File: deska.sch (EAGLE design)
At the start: 12 parts, among them IC1 78L05Z, T1 TIP122, T2 TIP122, T3 TIP122

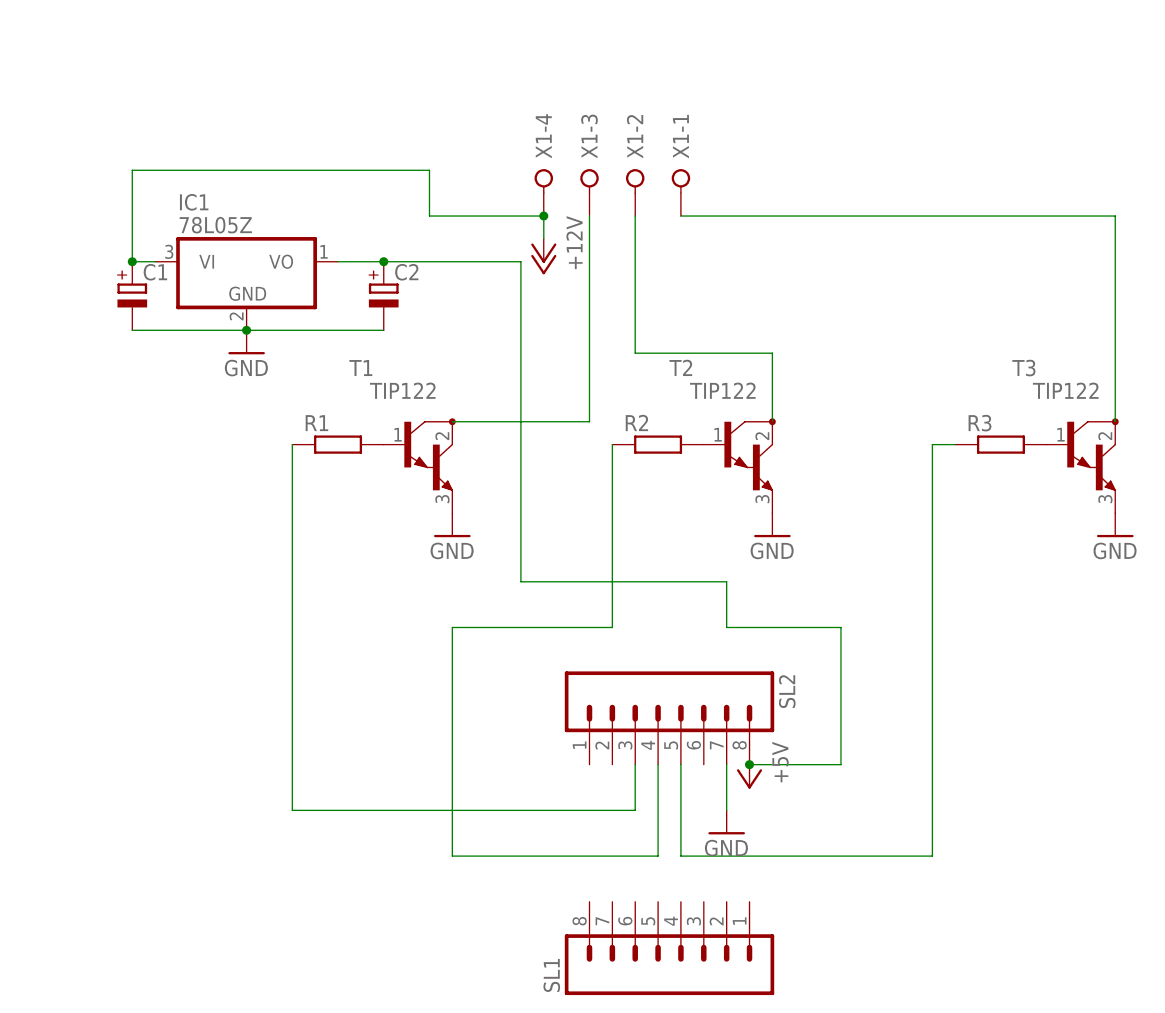
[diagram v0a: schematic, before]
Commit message: verze ESP8266-01
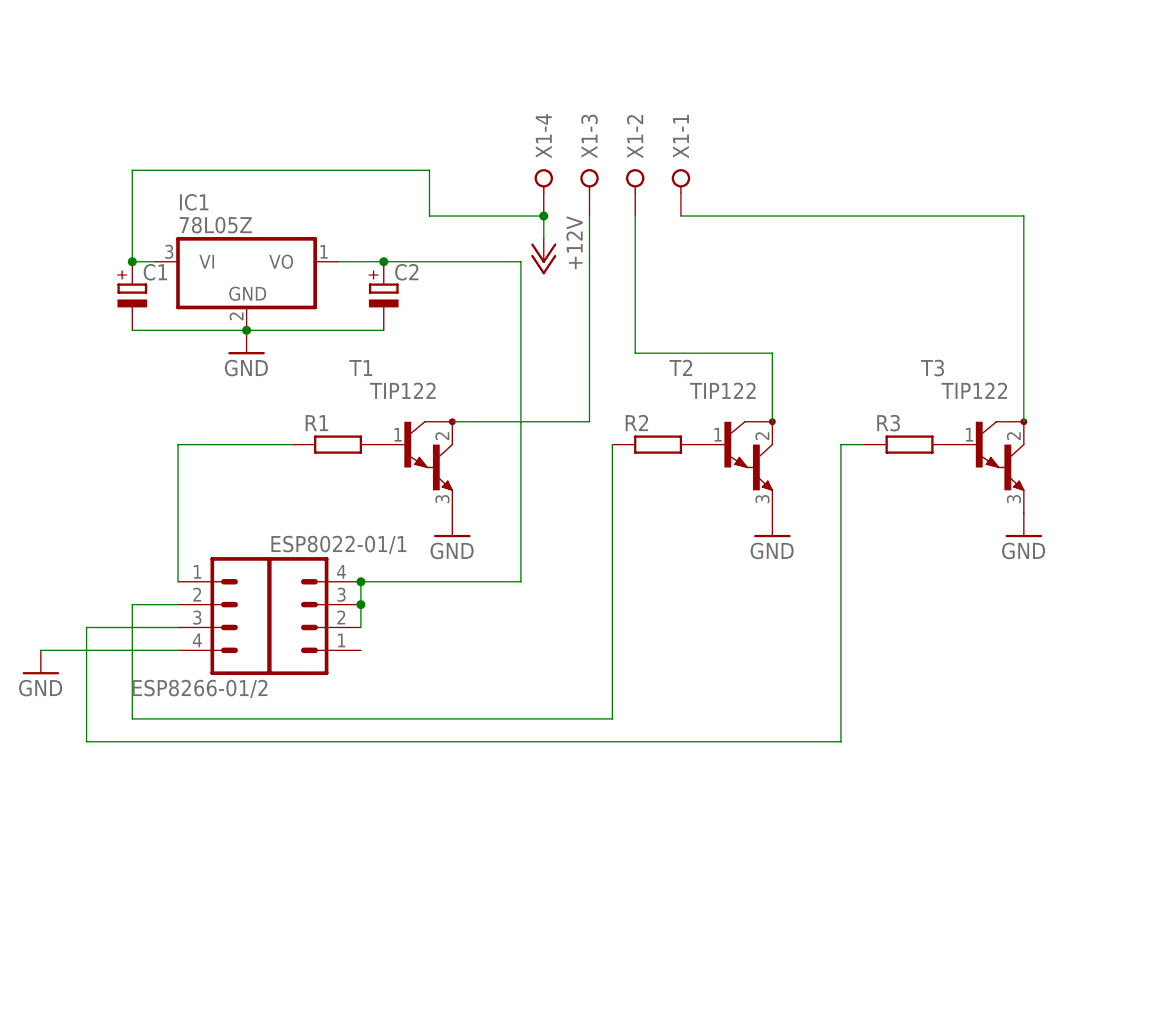
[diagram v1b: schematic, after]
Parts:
- removed SL1, SL2: (no value), con-amp-quick:M08
- added ESP8022-01/1, ESP8266-01/2: (no value), con-amp-quick:M04
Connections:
- removed net +5V: C2.+, IC1.VO, SL2.8
- removed net N$9: R3.1, SL2.5
- new net N$10: ESP8266-01/2.3, R3.1
- new net N$11: C2.+, ESP8022-01/1.2, ESP8022-01/1.3, ESP8022-01/1.4, IC1.VO
- net GND: now also ESP8266-01/2.4; no longer SL2.7
- net N$7: now also ESP8266-01/2.1; no longer SL2.3
- net N$8: now also ESP8266-01/2.2; no longer SL2.4
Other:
- moved on the sheet: R3, T3

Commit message: zmeny plosnaku
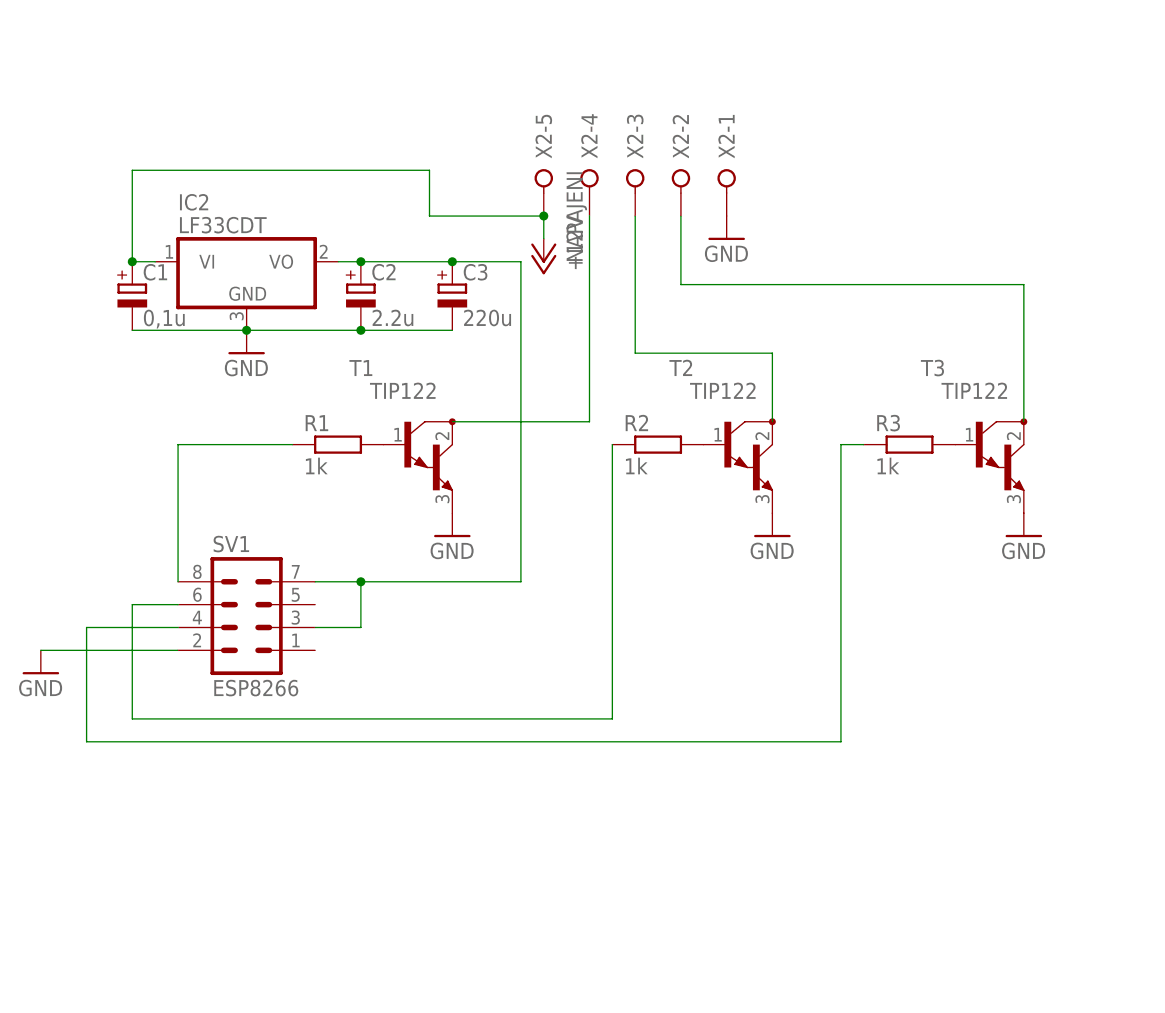
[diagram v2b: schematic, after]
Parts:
- removed ESP8022-01/1, ESP8266-01/2: (no value), con-amp-quick:M04
- removed IC1: 78L05Z, linear:78L05Z
- removed X1: (no value), con-wago-508:W237-04P
- added C3: 220u, rcl:CPOL-EUE3.5-8
- added IC2: LF33CDT, linear:7805DT
- added SV1: ESP8266, con-lstb:MA04-2
- added X2: NAPAJENI, con-wago-508:W237-05P
- C1: value (none) -> 0,1u
- C2: value (none) -> 2.2u
- R1, R2, R3: value (none) -> 1k
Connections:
- net +12V: now also IC2.VI, X2-5.KL; no longer IC1.VI, X1-4.KL
- net GND: now also C3.-, IC2.GND, SV1.2, X2-1.KL; no longer ESP8266-01/2.4, IC1.GND
- net N$1: now also X2-4.KL; no longer X1-3.KL
- net N$10: now also SV1.4; no longer ESP8266-01/2.3
- net N$11: now also C3.+, IC2.VO, SV1.3, SV1.7; no longer ESP8022-01/1.2, ESP8022-01/1.3, ESP8022-01/1.4, IC1.VO
- net N$2: now also X2-3.KL; no longer X1-2.KL
- net N$3: now also X2-2.KL; no longer X1-1.KL
- net N$7: now also SV1.8; no longer ESP8266-01/2.1
- net N$8: now also SV1.6; no longer ESP8266-01/2.2
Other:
- moved on the sheet: C2

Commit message: uprava desky
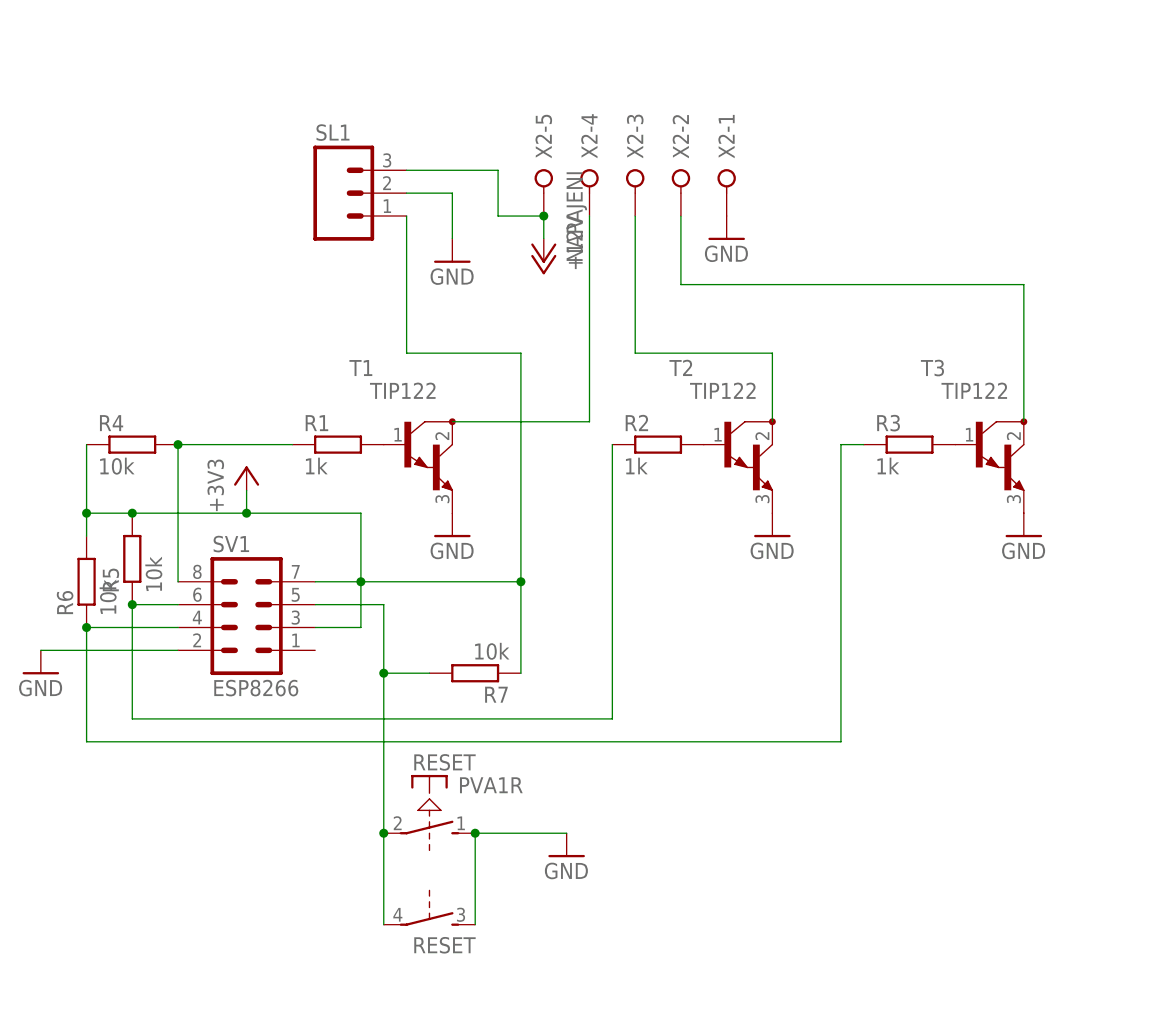
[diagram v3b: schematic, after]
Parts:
- removed C1: 0,1u, rcl:CPOL-EUE2-5
- removed C2: 2.2u, rcl:CPOL-EUE2-5
- removed C3: 220u, rcl:CPOL-EUE3.5-8
- removed IC2: LF33CDT, linear:7805DT
- added R4, R5, R6, R7: 10k, rcl:R-EU_0207/10
- added RESET: PVA1R, switch-misc:PVA1R
- added SL1: (no value), con-amp-quick:M03
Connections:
- removed net N$11: C2.+, C3.+, IC2.VO, SV1.3, SV1.7
- new net +3V3: R4.1, R5.2, R6.2, R7.1, SL1.1, SV1.3, SV1.7
- new net N$12: R7.2, RESET1.P, RESET2.P, SV1.5
- net +12V: now also SL1.3; no longer C1.+, IC2.VI
- net GND: now also RESET1.S, RESET2.S, SL1.2; no longer C1.-, C2.-, C3.-, IC2.GND
- net N$10: now also R6.1
- net N$7: now also R4.2
- net N$8: now also R5.1
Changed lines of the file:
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@@
 <?xml version="1.0" encoding="utf-8"?>
 <!DOCTYPE eagle SYSTEM "eagle.dtd">
-<eagle version="7.7.0">
+<eagle version="9.1.3">
 <drawing>
 <settings>
 <setting alwaysvectorfont="no"/>
+<setting keepoldvectorfont="yes"/>
 <setting verticaltext="up"/>
 </settings>
@@
 <part name="R2" library="rcl" deviceset="R-EU_" device="0207/10" value="1k"/>
 <part name="R3" library="rcl" deviceset="R-EU_" device="0207/10" value="1k"/>
-<part name="GND5" library="supply1" deviceset="GND" device=""/>
 <part name="GND6" library="supply1" deviceset="GND" device=""/>
-<part name="C3" library="rcl" deviceset="CPOL-EU" device="E3.5-8" value="220u"/>
-<part name="IC2" library="linear" deviceset="78*" device="DT" technology="05" value="LF33CDT"/>
 <part name="X2" library="con-wago-508" deviceset="W237-05P" device="" value="NAPAJENI"/>
 <part name="GND4" library="supply1" deviceset="GND" device=""/>
-<part name="C1" library="rcl" deviceset="CPOL-EU" device="E2-5" value="0,1u"/>
-<part name="C2" library="rcl" deviceset="CPOL-EU" device="E2-5" value="2.2u"/>
 <part name="SV1" library="con-lstb" deviceset="MA04-2" device="" value="ESP8266"/>
+<part name="R4" library="rcl" deviceset="R-EU_" device="0207/10" value="10k"/>
+<part name="R5" library="rcl" deviceset="R-EU_" device="0207/10" value="10k"/>
+<part name="R6" library="rcl" deviceset="R-EU_" device="0207/10" value="10k"/>
+<part name="R7" library="rcl" deviceset="R-EU_" device="0207/10" value="10k"/>
+<part name="RESET" library="switch-misc" library_urn="urn:adsk.eagle:library:376" deviceset="PVA1R" device="" package3d_urn="urn:adsk.eagle:package:27429/1"/>
+<part name="GND7" library="supply1" deviceset="GND" device=""/>
+<part name="+3V1" library="supply1" library_urn="urn:adsk.eagle:library:371" deviceset="+3V3" device=""/>
+<part name="SL1" library="con-amp-quick" library_urn="urn:adsk.eagle:library:125" deviceset="M03" device="" package3d_urn="urn:adsk.eagle:package:5957/1"/>
+<part name="GND5" library="supply1" deviceset="GND" device=""/>
 </parts>
 <sheets>
@@
 <instance part="R2" gate="G$1" x="45.72" y="66.04"/>
 <instance part="R3" gate="G$1" x="73.66" y="66.04"/>
-<instance part="GND5" gate="1" x="0" y="76.2"/>
 <instance part="GND6" gate="1" x="-22.86" y="40.64"/>
-<instance part="C3" gate="G$1" x="22.86" y="83.82"/>
-<instance part="IC2" gate="A1" x="0" y="86.36"/>
 <instance part="X2" gate="-1" x="53.34" y="96.52" rot="R270"/>
 <instance part="X2" gate="-2" x="48.26" y="96.52" rot="R270"/>
@@
 <instance part="X2" gate="-5" x="33.02" y="96.52" rot="R270"/>
 <instance part="GND4" gate="1" x="53.34" y="88.9"/>
-<instance part="C1" gate="G$1" x="-12.7" y="83.82"/>
-<instance part="C2" gate="G$1" x="12.7" y="83.82"/>
 <instance part="SV1" gate="G$1" x="0" y="48.26"/>
+<instance part="R4" gate="G$1" x="-12.7" y="66.04"/>
+<instance part="R5" gate="G$1" x="-12.7" y="53.34" rot="R90"/>
+<instance part="R6" gate="G$1" x="-17.78" y="50.8" rot="R90"/>
+<instance part="R7" gate="G$1" x="25.4" y="40.64" rot="R180"/>
+<instance part="RESET" gate="1" x="20.32" y="22.86" rot="R270"/>
+<instance part="RESET" gate="2" x="20.32" y="12.7" rot="R270"/>
+<instance part="GND7" gate="1" x="35.56" y="20.32"/>
+<instance part="+3V1" gate="G$1" x="0" y="63.5"/>
+<instance part="SL1" gate="G$1" x="10.16" y="93.98"/>
+<instance part="GND5" gate="1" x="22.86" y="86.36"/>
 </instances>
 <busses>
@@
 </segment>
 <segment>
-<pinref part="GND5" gate="1" pin="GND"/>
-<wire x1="-12.7" y1="78.74" x2="0" y2="78.74" width="0.1524" layer="91"/>
-<junction x="0" y="78.74"/>
-<wire x1="0" y1="78.74" x2="12.7" y2="78.74" width="0.1524" layer="91"/>
-<pinref part="C3" gate="G$1" pin="-"/>
-<pinref part="IC2" gate="A1" pin="GND"/>
-<pinref part="C1" gate="G$1" pin="-"/>
-<pinref part="C2" gate="G$1" pin="-"/>
-<wire x1="12.7" y1="78.74" x2="22.86" y2="78.74" width="0.1524" layer="91"/>
-<junction x="12.7" y="78.74"/>
-</segment>
-<segment>
 <pinref part="GND6" gate="1" pin="GND"/>
 <wire x1="-22.86" y1="43.18" x2="-7.62" y2="43.18" width="0.1524" layer="91"/>
@@
 <pinref part="GND4" gate="1" pin="GND"/>
 </segment>
+<segment>
+<pinref part="RESET" gate="1" pin="S"/>
+<pinref part="RESET" gate="2" pin="S"/>
+<wire x1="25.4" y1="22.86" x2="25.4" y2="12.7" width="0.1524" layer="91"/>
+<wire x1="25.4" y1="22.86" x2="35.56" y2="22.86" width="0.1524" layer="91"/>
+<junction x="25.4" y="22.86"/>
+<pinref part="GND7" gate="1" pin="GND"/>
+</segment>
+<segment>
+<pinref part="SL1" gate="G$1" pin="2"/>
+<pinref part="GND5" gate="1" pin="GND"/>
+<wire x1="17.78" y1="93.98" x2="22.86" y2="93.98" width="0.1524" layer="91"/>
+<wire x1="22.86" y1="93.98" x2="22.86" y2="88.9" width="0.1524" layer="91"/>
+</segment>
 </net>
 <net name="+12V" class="0">
@@
 <pinref part="P+1" gate="1" pin="+12V"/>
 <wire x1="33.02" y1="88.9" x2="33.02" y2="91.44" width="0.1524" layer="91"/>
-<wire x1="-10.16" y1="86.36" x2="-12.7" y2="86.36" width="0.1524" layer="91"/>
-<wire x1="-12.7" y1="86.36" x2="-12.7" y2="96.52" width="0.1524" layer="91"/>
-<wire x1="-12.7" y1="96.52" x2="20.32" y2="96.52" width="0.1524" layer="91"/>
-<wire x1="20.32" y1="96.52" x2="20.32" y2="91.44" width="0.1524" layer="91"/>
-<wire x1="20.32" y1="91.44" x2="33.02" y2="91.44" width="0.1524" layer="91"/>
-<pinref part="IC2" gate="A1" pin="VI"/>
 <pinref part="X2" gate="-5" pin="KL"/>
+<pinref part="SL1" gate="G$1" pin="3"/>
+<wire x1="17.78" y1="96.52" x2="27.94" y2="96.52" width="0.1524" layer="91"/>
+<wire x1="27.94" y1="96.52" x2="27.94" y2="91.44" width="0.1524" layer="91"/>
+<wire x1="27.94" y1="91.44" x2="33.02" y2="91.44" width="0.1524" layer="91"/>
 <junction x="33.02" y="91.44"/>
-<pinref part="C1" gate="G$1" pin="+"/>
-<junction x="-12.7" y="86.36"/>
 </segment>
 </net>
@@
 <wire x1="-7.62" y1="66.04" x2="5.08" y2="66.04" width="0.1524" layer="91"/>
 <pinref part="SV1" gate="G$1" pin="8"/>
+<pinref part="R4" gate="G$1" pin="2"/>
+<junction x="-7.62" y="66.04"/>
 </segment>
 </net>
@@
 <wire x1="-12.7" y1="35.56" x2="40.64" y2="35.56" width="0.1524" layer="91"/>
 <pinref part="SV1" gate="G$1" pin="6"/>
+<pinref part="R5" gate="G$1" pin="1"/>
+<junction x="-12.7" y="48.26"/>
 </segment>
 </net>
@@
 <wire x1="66.04" y1="33.02" x2="66.04" y2="66.04" width="0.1524" layer="91"/>
 <pinref part="SV1" gate="G$1" pin="4"/>
-</segment>
-</net>
-<net name="N$11" class="0">
-<segment>
-<wire x1="10.16" y1="86.36" x2="12.7" y2="86.36" width="0.1524" layer="91"/>
-<wire x1="12.7" y1="86.36" x2="22.86" y2="86.36" width="0.1524" layer="91"/>
-<wire x1="22.86" y1="86.36" x2="30.48" y2="86.36" width="0.1524" layer="91"/>
-<wire x1="30.48" y1="86.36" x2="30.48" y2="50.8" width="0.1524" layer="91"/>
+<pinref part="R6" gate="G$1" pin="1"/>
+<junction x="-17.78" y="45.72"/>
+</segment>
+</net>
+<net name="N$12" class="0">
+<segment>
+<pinref part="RESET" gate="1" pin="P"/>
+<pinref part="RESET" gate="2" pin="P"/>
+<wire x1="15.24" y1="22.86" x2="15.24" y2="12.7" width="0.1524" layer="91"/>
+<wire x1="15.24" y1="22.86" x2="15.24" y2="40.64" width="0.1524" layer="91"/>
+<junction x="15.24" y="22.86"/>
+<pinref part="SV1" gate="G$1" pin="5"/>
+<pinref part="R7" gate="G$1" pin="2"/>
+<wire x1="7.62" y1="48.26" x2="15.24" y2="48.26" width="0.1524" layer="91"/>
+<wire x1="15.24" y1="48.26" x2="15.24" y2="40.64" width="0.1524" layer="91"/>
+<wire x1="15.24" y1="40.64" x2="20.32" y2="40.64" width="0.1524" layer="91"/>
+<junction x="15.24" y="40.64"/>
+</segment>
+</net>
+<net name="+3V3" class="0">
+<segment>
 <wire x1="30.48" y1="50.8" x2="12.7" y2="50.8" width="0.1524" layer="91"/>
-<pinref part="C3" gate="G$1" pin="+"/>
-<junction x="22.86" y="86.36"/>
-<pinref part="IC2" gate="A1" pin="VO"/>
-<pinref part="C2" gate="G$1" pin="+"/>
-<junction x="12.7" y="86.36"/>
 <pinref part="SV1" gate="G$1" pin="7"/>
 <pinref part="SV1" gate="G$1" pin="3"/>
@@
 <wire x1="12.7" y1="45.72" x2="12.7" y2="50.8" width="0.1524" layer="91"/>
 <junction x="12.7" y="50.8"/>
+<wire x1="12.7" y1="50.8" x2="12.7" y2="58.42" width="0.1524" layer="91"/>
+<pinref part="R6" gate="G$1" pin="2"/>
+<pinref part="R4" gate="G$1" pin="1"/>
+<wire x1="-17.78" y1="55.88" x2="-17.78" y2="58.42" width="0.1524" layer="91"/>
+<pinref part="R5" gate="G$1" pin="2"/>
+<wire x1="-17.78" y1="58.42" x2="-17.78" y2="66.04" width="0.1524" layer="91"/>
+<wire x1="-12.7" y1="58.42" x2="-17.78" y2="58.42" width="0.1524" layer="91"/>
+<junction x="-17.78" y="58.42"/>
+<wire x1="12.7" y1="58.42" x2="0" y2="58.42" width="0.1524" layer="91"/>
+<junction x="-12.7" y="58.42"/>
+<pinref part="R7" gate="G$1" pin="1"/>
+<wire x1="0" y1="58.42" x2="-12.7" y2="58.42" width="0.1524" layer="91"/>
+<wire x1="30.48" y1="50.8" x2="30.48" y2="40.64" width="0.1524" layer="91"/>
+<pinref part="+3V1" gate="G$1" pin="+3V3"/>
+<wire x1="0" y1="60.96" x2="0" y2="58.42" width="0.1524" layer="91"/>
+<junction x="0" y="58.42"/>
+<pinref part="SL1" gate="G$1" pin="1"/>
+<wire x1="17.78" y1="91.44" x2="17.78" y2="76.2" width="0.1524" layer="91"/>
+<wire x1="17.78" y1="76.2" x2="30.48" y2="76.2" width="0.1524" layer="91"/>
+<wire x1="30.48" y1="76.2" x2="30.48" y2="50.8" width="0.1524" layer="91"/>
+<junction x="30.48" y="50.8"/>
 </segment>
 </net>
@@
 </schematic>
 </drawing>
+<compatibility>
+<note version="8.2" severity="warning">
+Since Version 8.2, EAGLE supports online libraries. The ids
+of those online libraries will not be understood (or retained)
+with this version.
+</note>
+<note version="8.3" severity="warning">
+Since Version 8.3, EAGLE supports URNs for individual library
+assets (packages, symbols, and devices). The URNs of those assets
+will not be understood (or retained) with this version.
+</note>
+<note version="8.3" severity="warning">
+Since Version 8.3, EAGLE supports the association of 3D packages
+with devices in libraries, schematics, and board files. Those 3D
+packages will not be understood (or retained) with this version.
+</note>
+</compatibility>
 </eagle>
